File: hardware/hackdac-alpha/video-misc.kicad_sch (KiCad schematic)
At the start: 43 parts, among them J13 TTL SYNC, J2 SYNC OUT, P1 BANK2_AUX, Q1 BC847, Q2 BC857, Q3 BC857, Q7 2N7002, U16 74LVC1G125, U5 MCP47FEB22A1-E/ST, U6 74LVCH16T245, X1 ECS-TXO-3225-270-TR

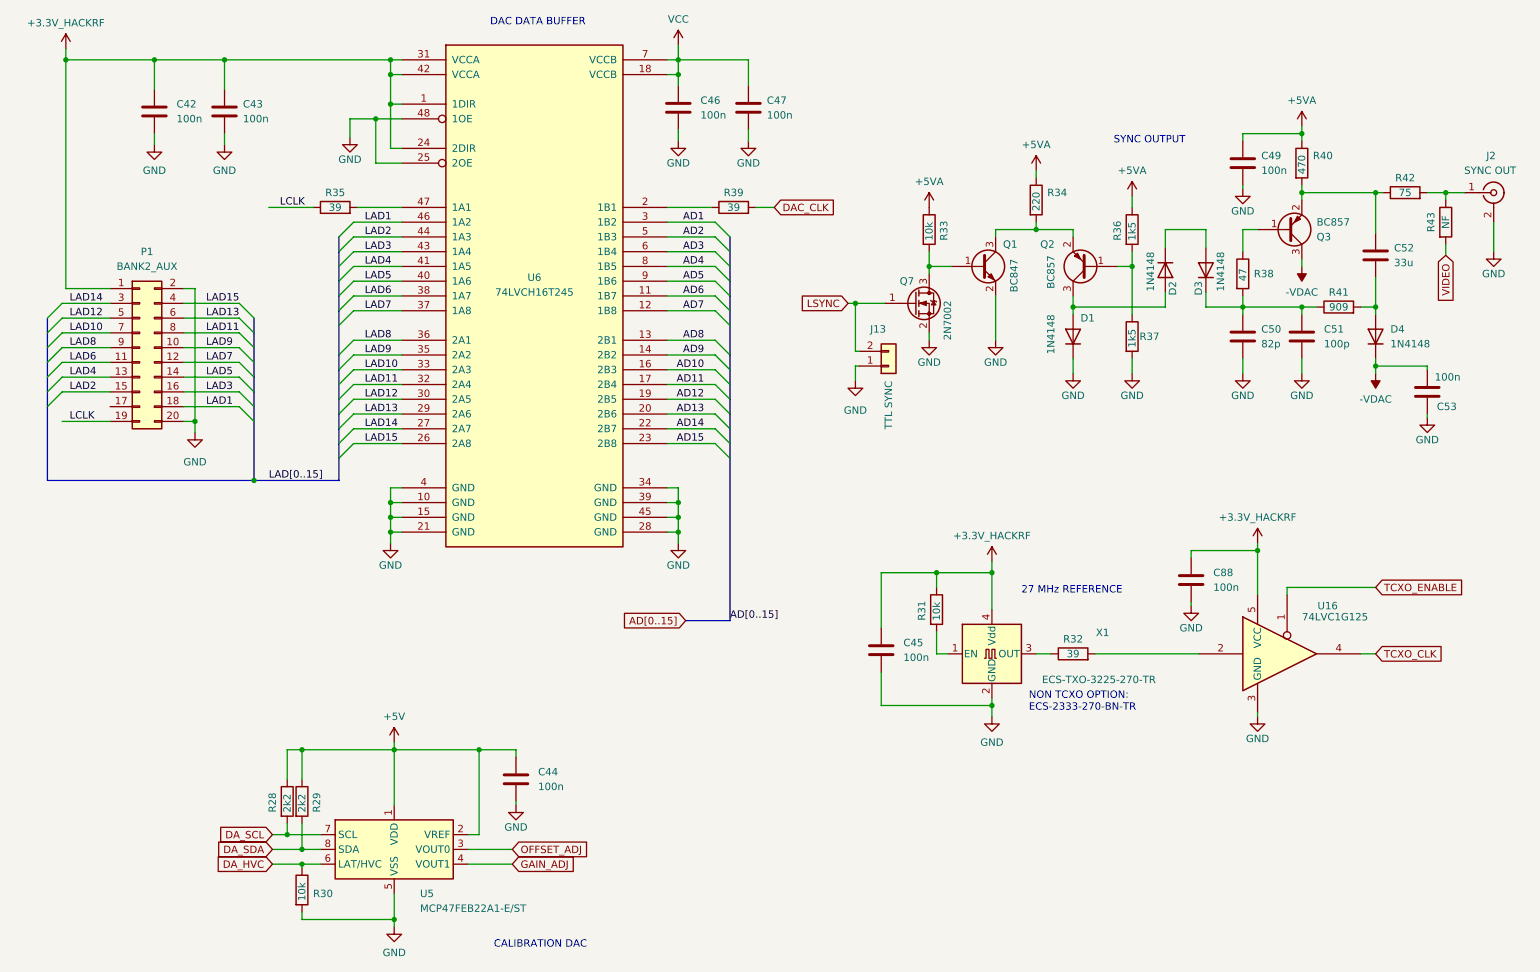
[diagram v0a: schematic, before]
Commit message: Last of major V3 changes
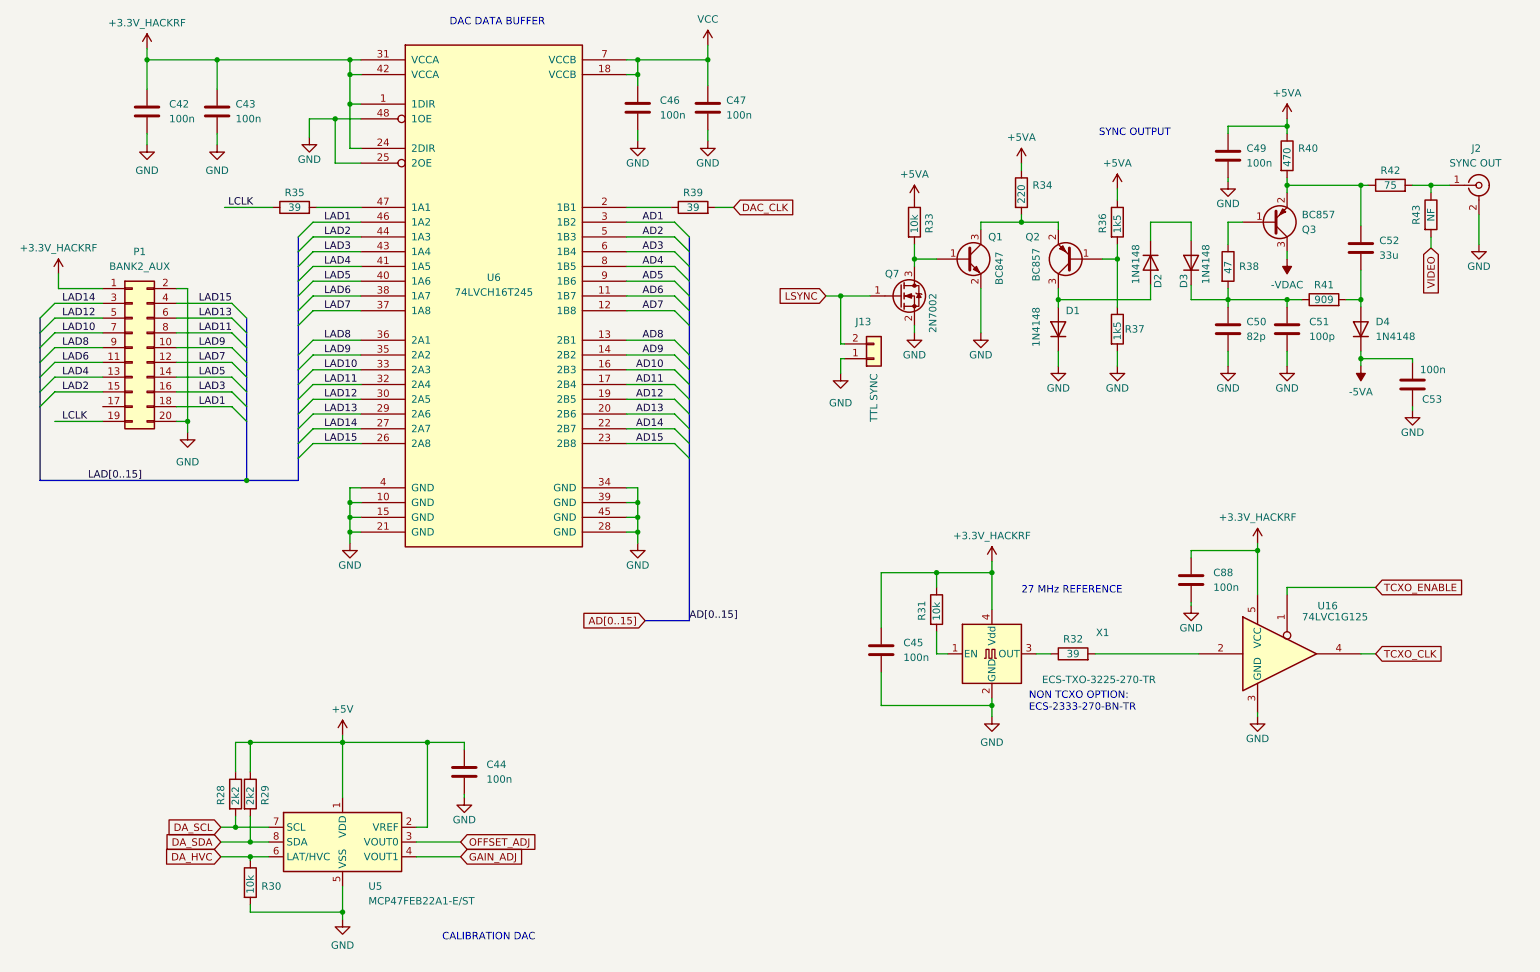
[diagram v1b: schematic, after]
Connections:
- net -VDAC: no longer C53.2, D4.1 (K)
- new net -5VA: C53.2, D4.1 (K)
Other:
- moved on the sheet: C42, C43, C44, C46, C47, C49, C50, C51, C52, C53, D1, D2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
